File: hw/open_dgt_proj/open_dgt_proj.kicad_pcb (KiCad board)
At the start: 2 copper layers, 1 part

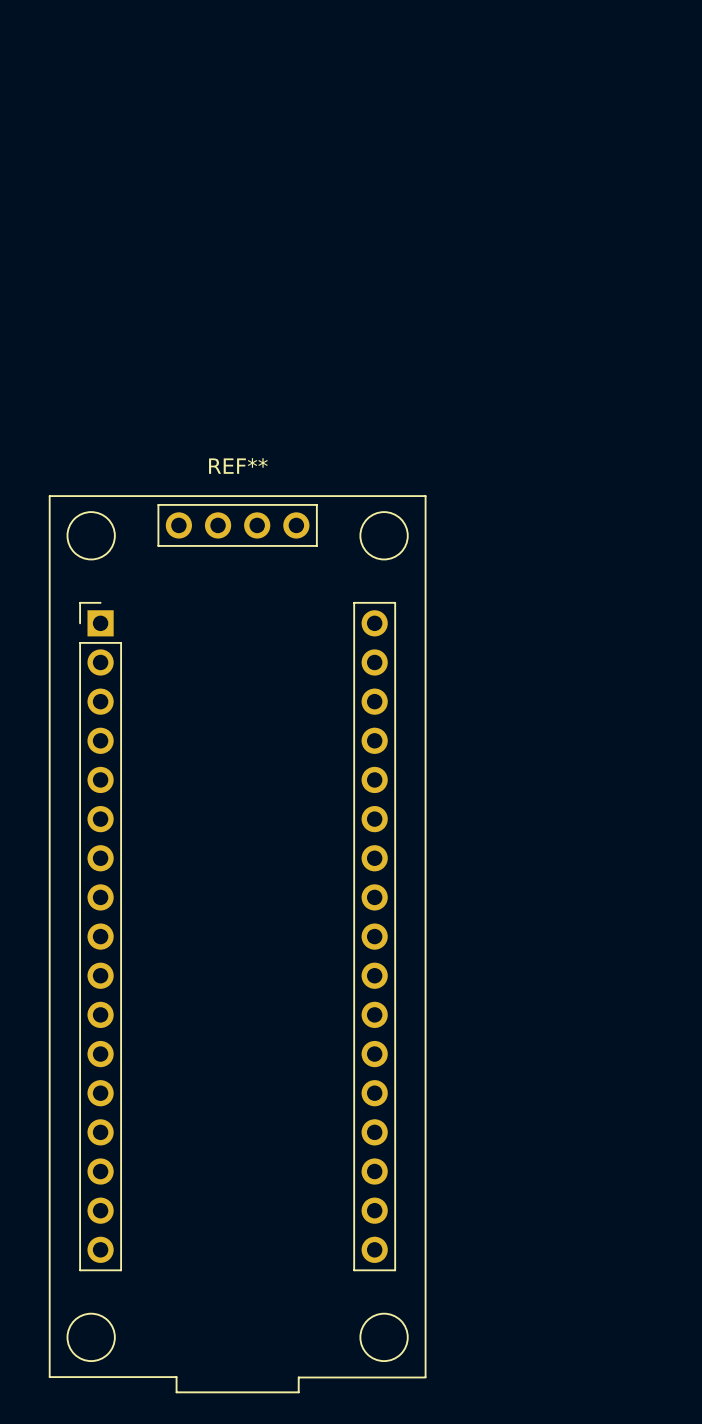
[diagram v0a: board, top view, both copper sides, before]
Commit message: Updated project schematic, PCB and 3D model
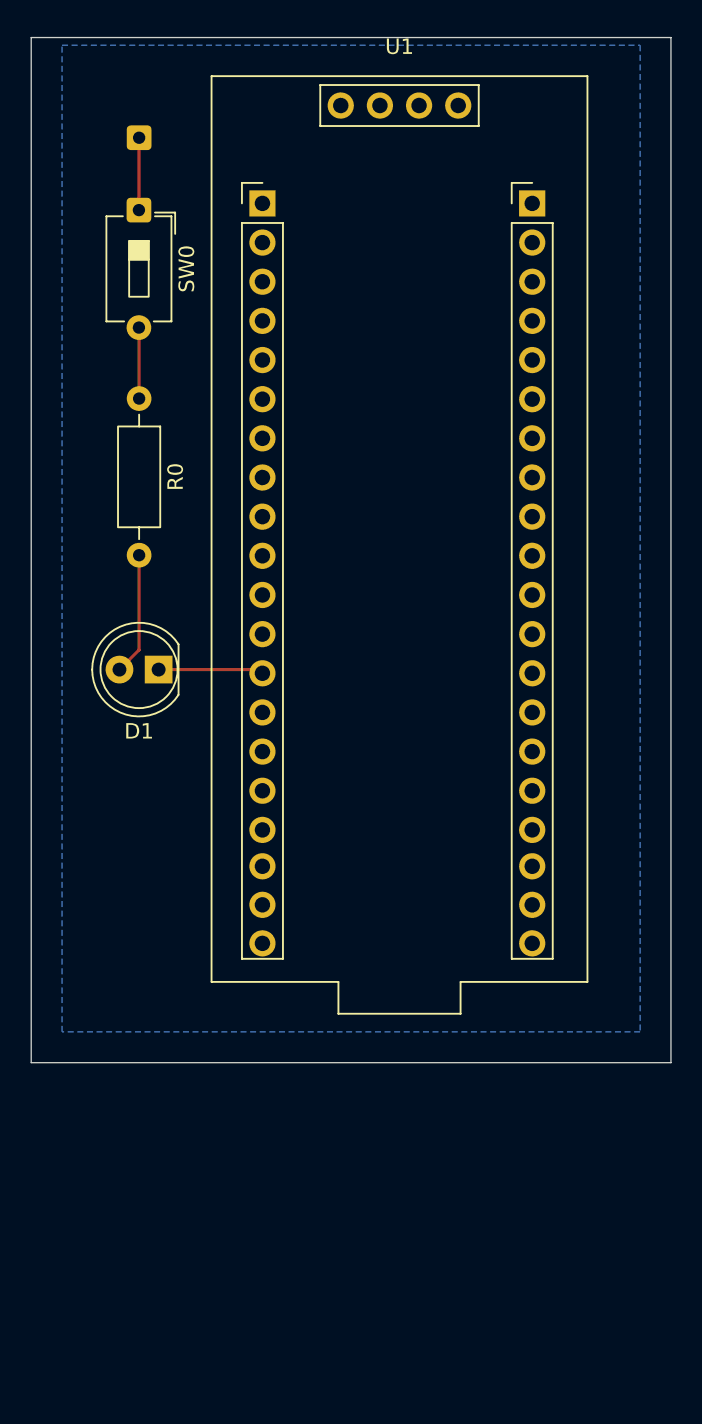
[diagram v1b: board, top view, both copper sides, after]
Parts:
- removed REF**: BlackPill, BlackPill_v2:YAAJ_BlackPill_SWD_2
- added ?: , , F.Cu at (135.0, 55.5)
- added D1: LED, LED_THT:LED_D5.0mm_FlatTop, F.Cu at (136.3, 90.0)
- added R0: 220, Resistor_THT:R_Axial_DIN0207_L6.3mm_D2.5mm_P10.16mm_Horizontal, F.Cu at (135.0, 72.4)
- added SW0: SW_DIP_x01, Button_Switch_THT:SW_DIP_SPSTx01_Slide_6.7x4.1mm_W7.62mm_P2.54mm_LowProfile, F.Cu at (135.0, 60.2)
- added U1: MiniF4-STM32F401CEU6, BlackPill_v2:YAAJ_BlackPill_SWD_2, F.Cu at (143.0, 59.8)
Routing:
- net Net-(D1-A): track 0.00 -> 7.95 mm
- net Net-(D1-K): track 0.00 -> 6.83 mm
- net /DGT0_SCL: track 0.00 -> 4.70 mm
- net Net-(R0-Pad1): track 0.00 -> 4.61 mm
- added copper zone on B.Cu, net GND
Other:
- board outline added: 41.5 x 66.5 mm
